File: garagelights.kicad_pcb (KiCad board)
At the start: 4 copper layers, 63.5 x 63.5 mm, 38 parts, among them J1 Conn_01x04, J2 Conn_01x06, J3 Screw_Terminal_01x01, J4 Screw_Terminal_01x01, Q1 ZVN4206AV, Q2 ZVN4206AV, Q3 ZVN4206AV, U1 NE555P, U2 NE555P, U3 4013, U4 LM7805_TO220, U5 4013

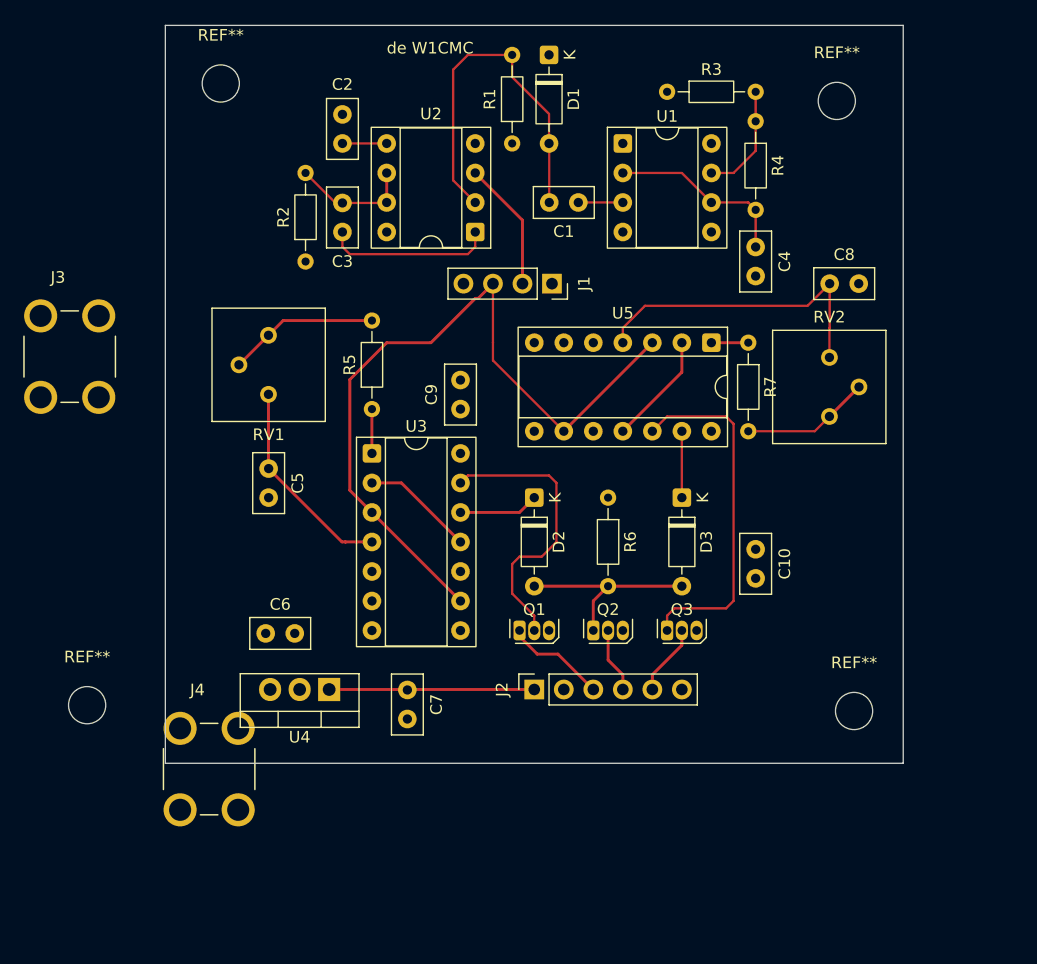
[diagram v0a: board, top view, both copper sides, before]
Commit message: Kinda sorta Rev_A
Finished the layout and brought it down to two layers, one of which
is a ground plane. Imported missing 3D models.
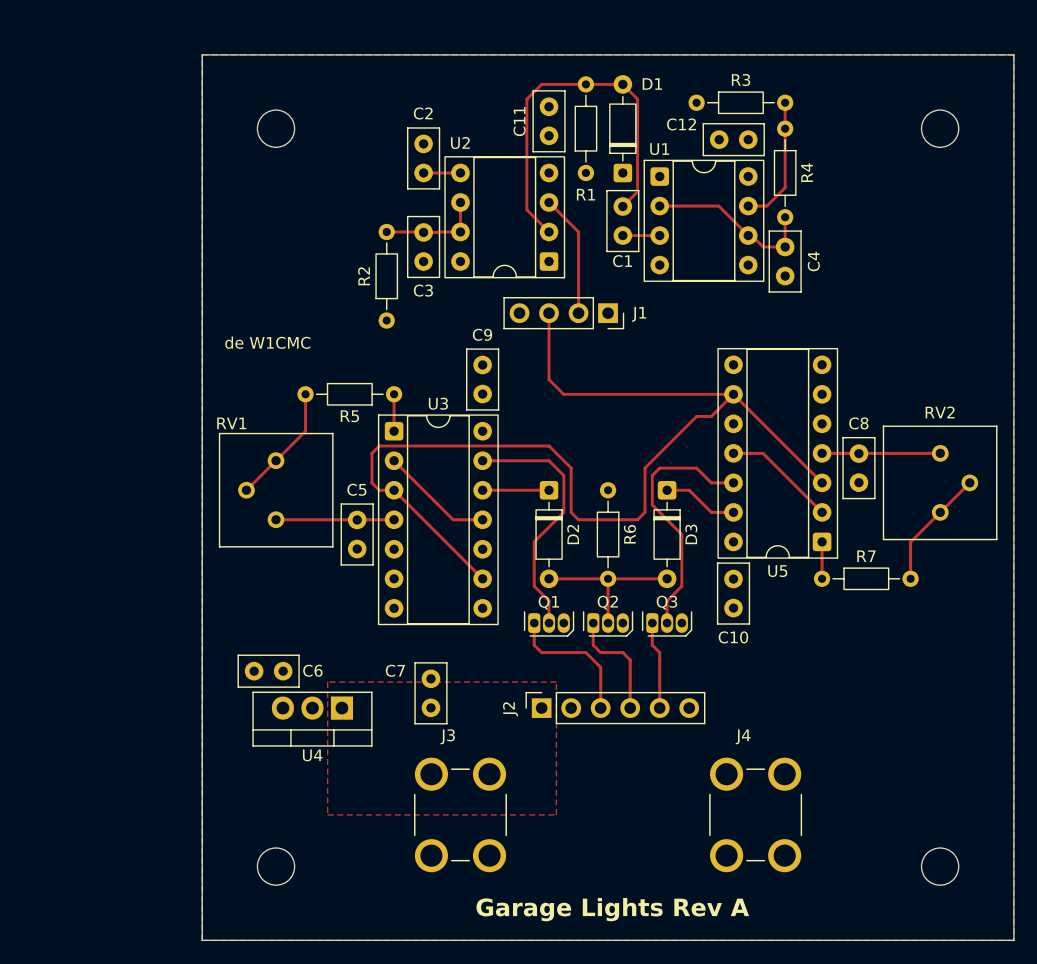
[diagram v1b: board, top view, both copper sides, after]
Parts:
- removed the REF** at (183.5, 70.0)
- removed the REF** at (185.0, 122.5)
- removed the REF** at (119.0, 122.0)
- removed the REF** at (130.5, 68.5)
- added C11: 0.1, Capacitor_THT:C_Disc_D5.0mm_W2.5mm_P2.50mm, F.Cu at (158.8, 73.0)
- added C12: 0.1, Capacitor_THT:C_Disc_D5.0mm_W2.5mm_P2.50mm, F.Cu at (175.9, 73.3)
- added REF**: MountingHole_3.2mm_M3, MountingHole:MountingHole_3.2mm_M3, F.Cu at (135.3, 135.9)
- added REF**: MountingHole_3.2mm_M3, MountingHole:MountingHole_3.2mm_M3, F.Cu at (192.4, 72.4)
- added REF**: MountingHole_3.2mm_M3, MountingHole:MountingHole_3.2mm_M3, F.Cu at (135.3, 72.4)
- added REF**: MountingHole_3.2mm_M3, MountingHole:MountingHole_3.2mm_M3, F.Cu at (192.4, 135.9)
- moved J3 51.8 mm to (151.1, 131.4)
- moved J4 47.2 mm to (176.5, 131.4)
- moved R7 21.3 mm to (182.2, 111.1), turned to 0 degrees
- moved U5 19.6 mm to (182.2, 108.0), turned to 180 degrees
- moved C8 14.8 mm to (185.4, 100.3), turned to -90 degrees
- moved RV2 12.6 mm to (192.4, 105.4)
- moved D1 12.0 mm to (165.1, 76.2), turned to 90 degrees
- moved RV1 10.8 mm to (135.3, 101.0)
- moved C5 8.81 mm to (142.2, 106.1)
- moved R2 8.64 mm to (144.8, 88.9)
- moved C2 7.43 mm to (148.0, 76.2)
- moved C3 7.43 mm to (148.0, 81.3)
- moved R1 6.84 mm to (161.9, 76.2)
- moved U2 6.84 mm to (158.8, 83.8)
- moved J1 5.45 mm to (163.8, 88.3)
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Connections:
- Q2 pad 1: Net-(D2-A) -> Net-(J2-Pin_4)
- Q2 pad 2: Net-(J2-Pin_4) -> Net-(D2-A)
- Q3 pad 1: Net-(Q3-G) -> Net-(J2-Pin_5)
- Q3 pad 2: Net-(J2-Pin_5) -> Net-(Q3-G)
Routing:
- net Net-(J1-Pin_3): track 64.7 -> 91.3 mm
- net +12V: track 17.7 -> 0.00 mm
- net Net-(U5A-R): track 27.0 -> 10.2 mm
- net GND: track 14.5 -> 0.00 mm
- net Net-(Q3-G): track 30.5 -> 22.1 mm
- net Net-(U3A-R): track 17.9 -> 10.2 mm
- net Net-(J2-Pin_4): track 5.61 -> 9.75 mm
- net Net-(Q1-G): track 25.0 -> 21.8 mm
- net Net-(J2-Pin_3): track 8.75 -> 11.9 mm
- net Net-(D2-A): track 17.0 -> 14.0 mm
- net Net-(R5-Pad2): track 13.0 -> 10.4 mm
- net Net-(U2-DIS): track 10.9 -> 9.29 mm
- net Net-(U1-DIS): track 9.68 -> 11.1 mm
- net Net-(J2-Pin_5): track 6.13 -> 7.58 mm
- net Net-(D2-K): track 6.88 -> 5.72 mm
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- added copper zone on F.Cu, net +12V
- added copper zone on F.Cu, net +5V
- added copper zone on B.Cu, net GND
- removed copper zone on In2.Cu, net +5V
- removed copper zone on In1.Cu, net GND
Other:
- board size 63.5 x 63.5 mm -> 69.8 x 76.2 mm
- copper layers 4 -> 2
- board text added: "Garage Lights Rev A"
